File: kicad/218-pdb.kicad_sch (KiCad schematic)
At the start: 65 parts, among them J1 Conn_01x03, J10 Conn_01x03, J11 Conn_01x03, J12 Conn_01x03, J13 Conn_01x03, J14 Conn_01x03, J15 Conn_01x03, J16 Conn_01x03, J17 Conn_01x03, J18 Conn_01x03, J19 Conn_01x03, J2 Conn_01x03, J20 Conn_01x03, J21 Conn_01x03, J22 Conn_01x03, J23 Conn_01x03, J24 Conn_01x03, J25 Conn_01x04_Pin, J26 Conn_01x04_Pin, J27 Conn_01x04_Pin, J28 Conn_01x04_Pin, J29 14 V molex, J3 Conn_01x03, J30 14 V molex, J31 14 V molex, J32 14 V molex, J33 external 5V, J34 battery, J35 battery, J4 Conn_01x03, J5 Conn_01x03, J6 Conn_01x03, J7 Conn_01x03, J8 Conn_01x03, J9 Conn_01x03, SW1 5V switch, U3 LD1117V33, U4 LD1117V33

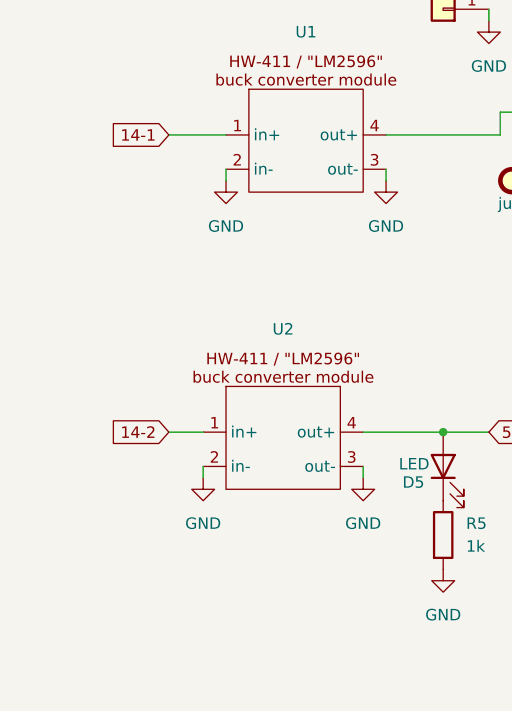
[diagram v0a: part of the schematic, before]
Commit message: update BOM, silkscreen
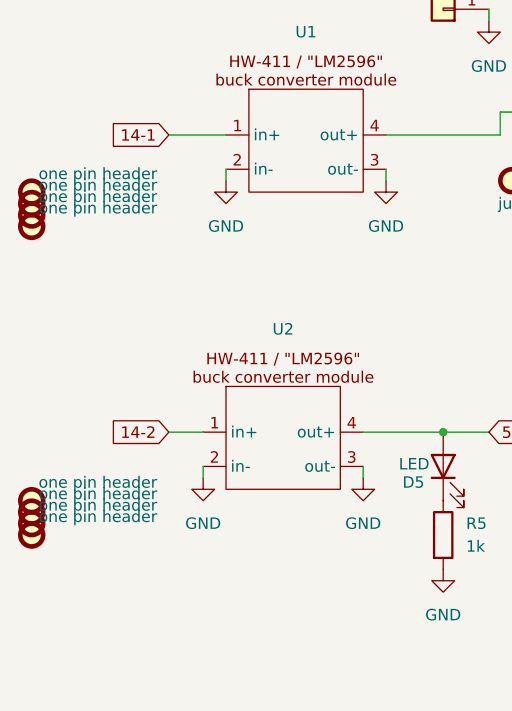
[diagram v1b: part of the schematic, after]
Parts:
- added FID10, FID3, FID4, FID5, FID6, FID7, FID8, FID9: one pin header, 218-pdb:PinHeader_1x01_P2.54mm_Vertical, symbol Mechanical:Fiducial
- D6: value D -> diode, >=1Amp; Part_Number (none) -> spdl, 1N4935
- U1, U2: value ~ -> DC-DC buck
- renumbered FID3 to FID2
